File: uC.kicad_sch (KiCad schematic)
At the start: 52 parts, among them J401 Conn_02x05_Counter_Clockwise, J402 Conn_02x05_Counter_Clockwise, J403 Conn_02x08_Counter_Clockwise, SW401 SW_Push, SW402 SW_Push, U401 STM32F103RGT6, U402 BLUENRG-M2SA, Y401 16MHz, Y402 32.768KHz

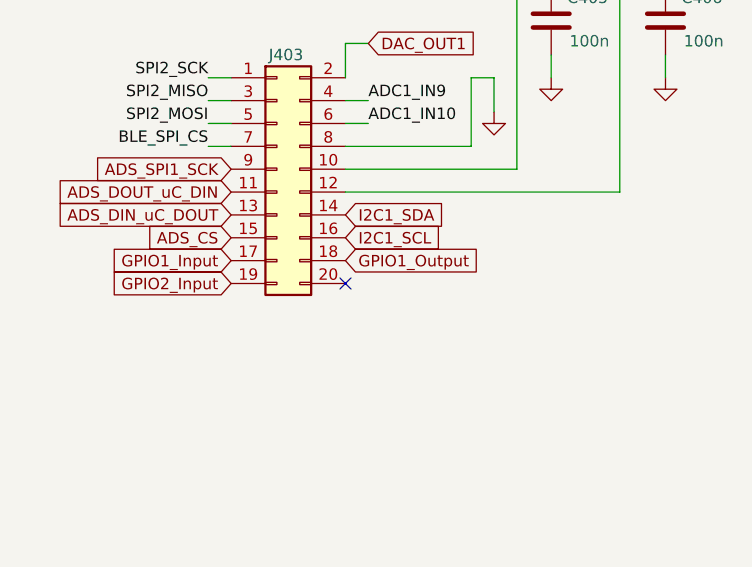
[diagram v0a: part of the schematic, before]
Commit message: all connections complete
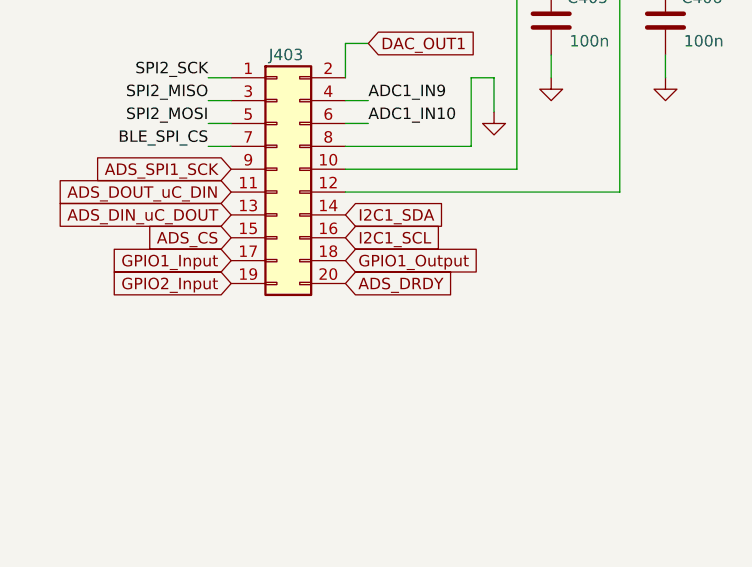
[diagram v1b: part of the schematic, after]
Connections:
- net ADS_DRDY: now also J403.20 (Pin_20)
- no-connect marks 17 -> 16
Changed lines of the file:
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@@
 	)
 	(no_connect
-		(at 360.68 153.67)
-	)
-	(no_connect
 		(at 78.74 193.04)
 	)
@@
 				(hide yes)
 			)
+		)
+	)
+	(global_label "ADS_DRDY"
+		(shape input)
+		(at 360.68 153.67 0)
+		(fields_autoplaced yes)
+		(effects
+			(font
+				(size 1.27 1.27)
+			)
+			(justify left)
+		)
+		(property "Intersheetrefs" "${INTERSHEET_REFS}"
+			(at 373.0995 153.67 0)
+			(effects
+				(font
+					(size 1.27 1.27)
+				)
+				(justify left)
+				(hide yes)
+			)
